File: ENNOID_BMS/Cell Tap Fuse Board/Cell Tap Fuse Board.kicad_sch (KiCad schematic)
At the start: 3 parts, among them J1 Conn_01x02

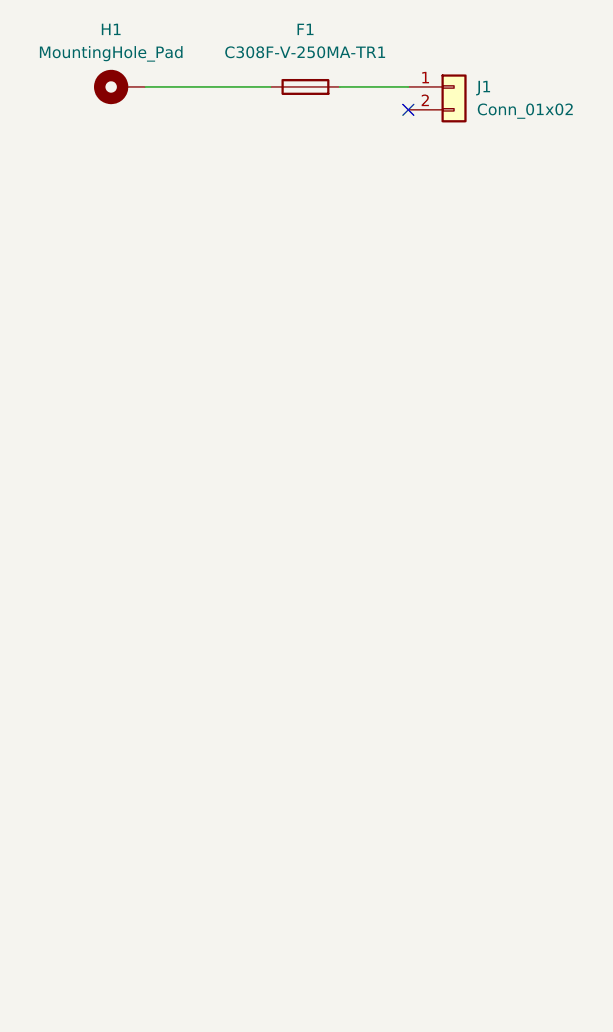
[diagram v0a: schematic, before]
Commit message: master and slave updated
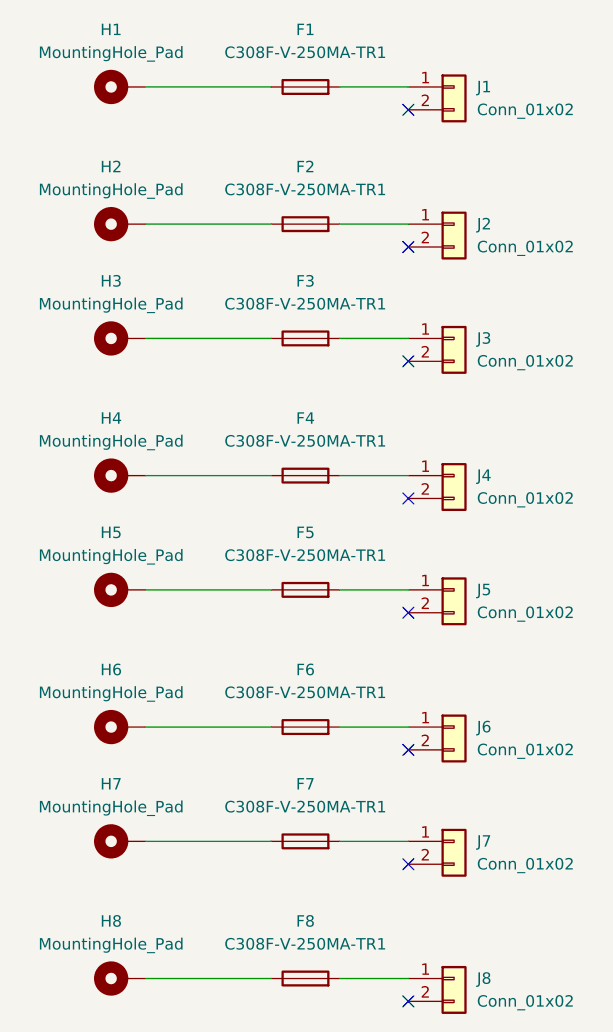
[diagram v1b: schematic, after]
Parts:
- added F2, F3, F4, F5, F6, F7, F8: C308F-V-250MA-TR1, Kicad_Libraries:C308F-V-250MA-TR1, symbol Device:Fuse
- added H2, H3, H4, H5, H6, H7, H8: MountingHole_Pad, MountingHole:MountingHole_5.5mm_Pad, symbol Mechanical:MountingHole_Pad
- added J2, J3, J4, J5, J6, J7, J8: Conn_01x02, Connector_Molex:Molex_PicoBlade_53047-0210_1x02_P1.25mm_Vertical, symbol Connector_Generic:Conn_01x02
- H1: footprint MountingHole:MountingHole_5.5mm_Pad_TopBottom -> MountingHole:MountingHole_5.5mm_Pad
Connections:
- new net: F8.1, H8.1
- new net: F7.2, J7.1 (Pin_1)
- new net: F4.1, H4.1
- new net: F4.2, J4.1 (Pin_1)
- new net: F6.1, H6.1
- new net: F6.2, J6.1 (Pin_1)
- new net: F7.1, H7.1
- new net: F8.2, J8.1 (Pin_1)
- new net: F2.2, J2.1 (Pin_1)
- new net: F3.1, H3.1
- new net: F3.2, J3.1 (Pin_1)
- new net: F5.1, H5.1
- new net: F5.2, J5.1 (Pin_1)
- new net: F2.1, H2.1
- no-connect marks 1 -> 8
